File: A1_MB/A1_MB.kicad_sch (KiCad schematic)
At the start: 12 parts, among them J1 Conn_02x04_Counter_Clockwise, J15 Conn_02x04_Odd_Even, J16 USB_A, J2 Screw_Terminal_01x02, U1 Pico

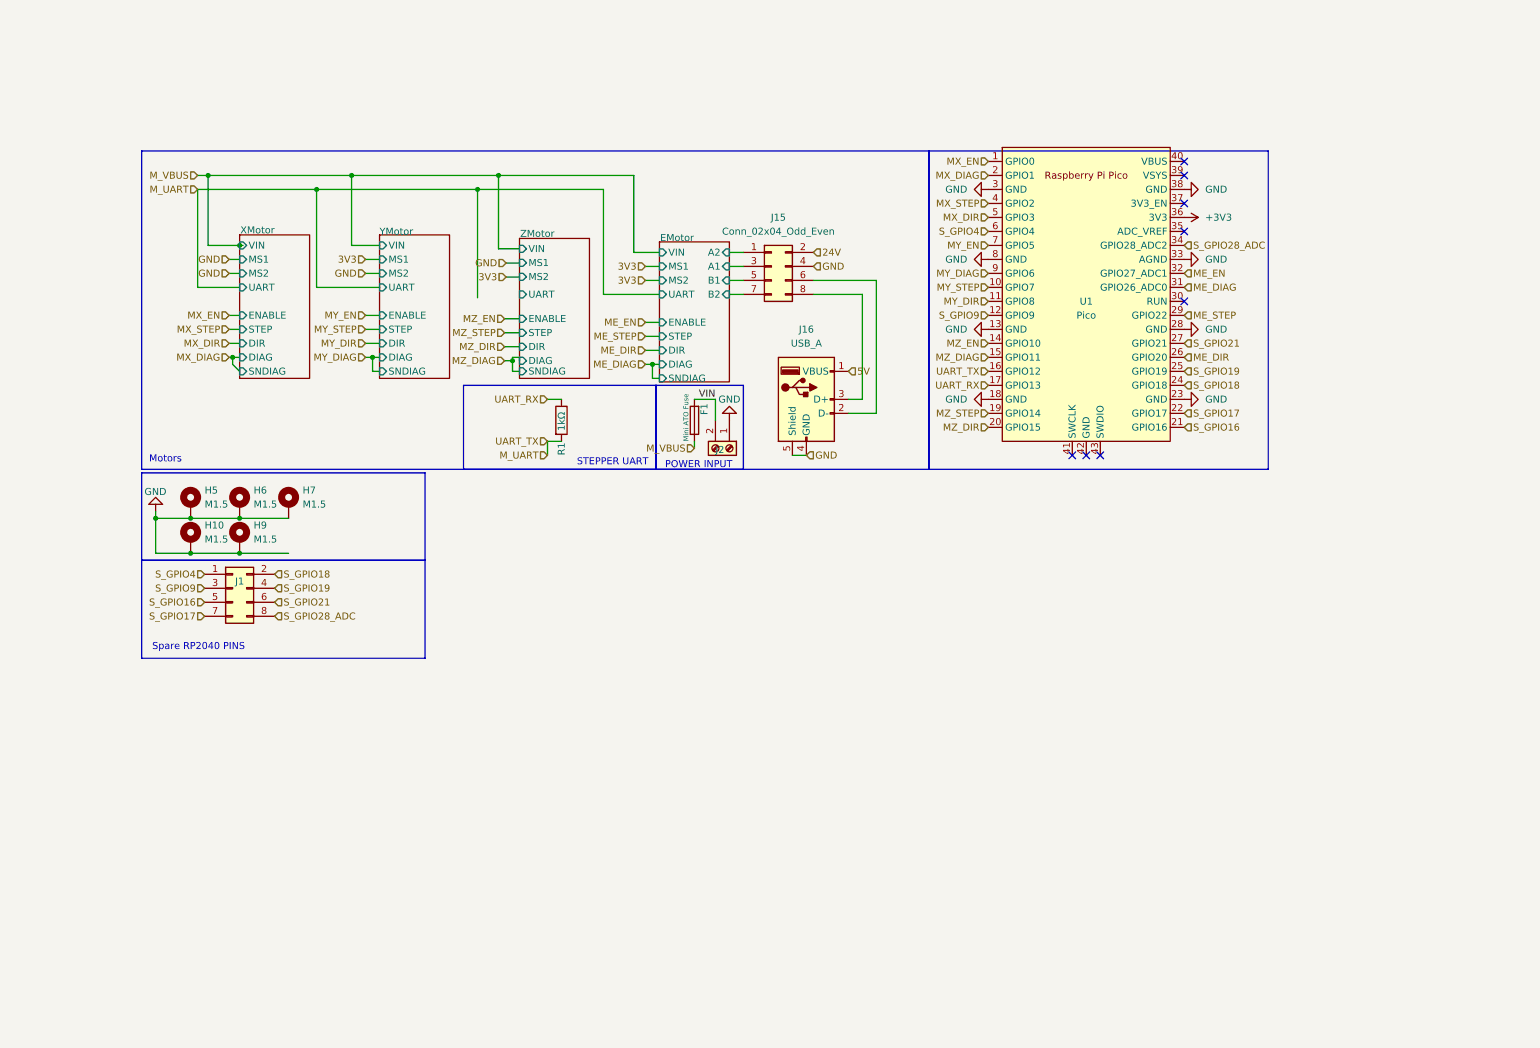
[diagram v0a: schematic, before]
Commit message: e
e
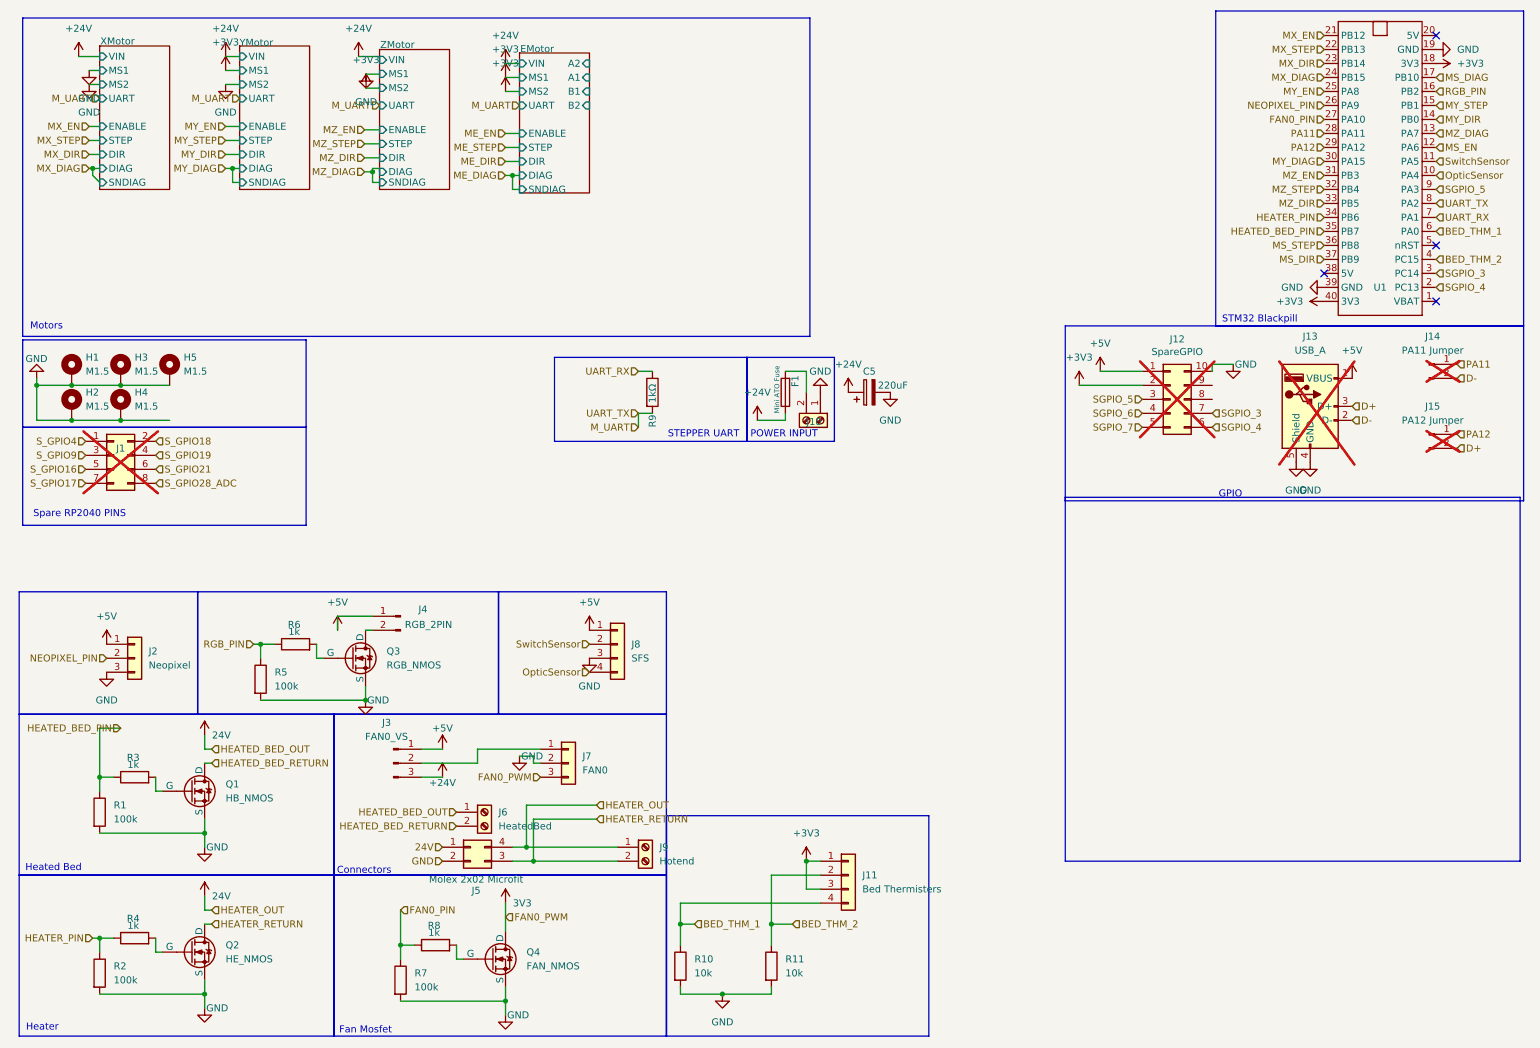
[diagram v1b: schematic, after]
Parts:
- removed J15: Conn_02x04_Odd_Even, symbol Connector_Generic:Conn_02x04_Odd_Even
- removed J16: USB_A, symbol Connector:USB_A
- removed U1: Pico, OpenA1K:Socketed MCU - Pico (No Text), symbol MCU_RaspberryPi_and_Boards:Pico
- added C5: 220uF, Capacitor_THT:CP_Radial_D8.0mm_P3.50mm, symbol Device:C_Polarized
- added J11: Bed Thermisters, Connector_JST:JST_XH_B4B-XH-A_1x04_P2.50mm_Vertical, symbol Connector_Generic:Conn_01x04
- added J12: SpareGPIO, Connector_PinHeader_2.54mm:PinHeader_2x05_P2.54mm_Vertical, symbol Connector_Generic:Conn_02x05_Counter_Clockwise
- added J13: USB_A, Connector_USB:USB3_A_Molex_48393-001, symbol Connector:USB_A
- added J14: PA11 Jumper, Connector_PinHeader_2.54mm:PinHeader_1x02_P2.54mm_Vertical, symbol Connector:Conn_01x02_Pin
- added J15: PA12 Jumper, Connector_PinHeader_2.54mm:PinHeader_1x02_P2.54mm_Vertical, symbol Connector:Conn_01x02_Pin
- added J2: Neopixel, Connector_JST:JST_XH_B3B-XH-AM_1x03_P2.50mm_Vertical, symbol Connector_Generic:Conn_01x03
- added J3: FAN0_VS, Connector_PinHeader_2.54mm:PinHeader_1x03_P2.54mm_Vertical, symbol Connector:Conn_01x03_Pin
- added J4: RGB_2PIN, Connector_JST:JST_XH_B2B-XH-AM_1x02_P2.50mm_Vertical, symbol Connector:Conn_01x02_Pin
- added J5: Molex 2x02 Microfit, Connector_Molex:Molex_Micro-Fit_3.0_43045-0412_2x02_P3.00mm_Vertical, symbol Connector_Generic:Conn_02x02_Counter_Clockwise
- added J6: HeatedBed, OpenA1K:ScrewTerminal 7mm x 7mm, symbol Connector:Screw_Terminal_01x02
- added J7: FAN0, Connector_JST:JST_XH_B3B-XH-AM_1x03_P2.50mm_Vertical, symbol Connector_Generic:Conn_01x03
- added J8: SFS, Connector_JST:JST_XH_B4B-XH-AM_1x04_P2.50mm_Vertical, symbol Connector_Generic:Conn_01x04
- added J9: Hotend, OpenA1K:ScrewTerminal 7mm x 7mm, symbol Connector:Screw_Terminal_01x02
- added Q1: HB_NMOS, OpenA1K:TO254P1054X469X1930-3, symbol Simulation_SPICE:NMOS
- added Q2: HE_NMOS, OpenA1K:TO254P1054X469X1930-3, symbol Simulation_SPICE:NMOS
- added Q3: RGB_NMOS, OpenA1K:TO254P1054X469X1930-3, symbol Simulation_SPICE:NMOS
- added Q4: FAN_NMOS, OpenA1K:TO254P1054X469X1930-3, symbol Simulation_SPICE:NMOS
- added R1, R2, R5, R7: 100k, Resistor_THT:R_Axial_DIN0207_L6.3mm_D2.5mm_P10.16mm_Horizontal, symbol Device:R
- added R10, R11: 10k, Resistor_THT:R_Axial_DIN0207_L6.3mm_D2.5mm_P10.16mm_Horizontal, symbol Device:R
- added R3, R4, R6, R8: 1k, Resistor_THT:R_Axial_DIN0207_L6.3mm_D2.5mm_P10.16mm_Horizontal, symbol Device:R
- added U1: ~, OpenA1K:STM32 Blackpill Socketed, symbol CustomSymbols:STM32F401_Black_Pill
- J1: now not fitted; now left out of the parts list
- renumbered H5 to H1, H10 to H2, H6 to H3, H9 to H4, H7 to H5, J2 to J10, R1 to R9
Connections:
- net +3V3: now also J11.1 (Pin_1), J11.3 (Pin_3), J12.2 (Pin_2), U1.18 (3V3), U1.40 (3V3)
- net 24V: now also J5.1 (Pin_1), J5.4 (Pin_4), J6.1 (Pin_1), J9.1 (Pin_1)
- net 3V3: now also J7.3 (Pin_3), Q4.1 (D)
- net GND: now also C5.2, J12.10 (Pin_10), J13.4 (GND), J13.5 (Shield), J2.3 (Pin_3), J5.2 (Pin_2), J7.2 (Pin_2), J8.3 (Pin_3), Q1.3 (S), Q2.3 (S), Q3.3 (S), Q4.3 (S), R1.2, R10.2, R11.2, R2.2, R5.2, R7.2, U1.19 (GND), U1.39 (GND)
- net MX_DIAG: now also U1.24 (PB15)
- net MX_DIR: now also U1.23 (PB14)
- net MX_EN: now also U1.21 (PB12)
- net MX_STEP: now also U1.22 (PB13)
- net MY_DIAG: now also U1.30 (PA15)
- net MY_DIR: now also U1.14 (PB0)
- net MY_EN: now also U1.25 (PA8)
- net MY_STEP: now also U1.15 (PB1)
- net MZ_DIAG: now also U1.13 (PA7)
- net MZ_DIR: now also U1.33 (PB5)
- net MZ_EN: now also U1.31 (PB3)
- net MZ_STEP: now also U1.32 (PB4)
- net M_UART: now also U1.8 (PA2)
- net UART_RX: now also U1.7 (PA1)
- net M_VBUS renamed +24V
- net +24V: now also C5.1, J3.3 (Pin_3)
- net VIN: no longer names the net of F1.2, J10.2 (Pin_2)
- new net: Q2.2 (G), R4.2
- new net: J3.2 (Pin_2), J7.1 (Pin_1)
- new net: J4.2 (Pin_2), Q3.1 (D)
- new net: Q3.2 (G), R6.2
- new net: Q1.2 (G), R3.2
- new net: Q4.2 (G), R8.2
- new net  HEATED_BED_PIN: R1.1, R3.1
- new net +5V: J12.1 (Pin_1), J13.1 (VBUS), J2.1 (Pin_1), J3.1 (Pin_1), J4.1 (Pin_1), J8.1 (Pin_1)
- new net BED_THM_1: J11.4 (Pin_4), R10.1, U1.6 (PA0)
- new net BED_THM_2: J11.2 (Pin_2), R11.1, U1.4 (PC15)
- new net D+: J13.3 (D+), J15.2 (Pin_2)
- new net D-: J13.2 (D-), J14.2 (Pin_2)
- new net FAN0_PIN: R7.1, R8.1, U1.27 (PA10)
- new net HEATED_BED_PIN: U1.35 (PB7)
- new net HEATED_BED_RETURN: J6.2 (Pin_2), Q1.1 (D)
- new net HEATER_PIN: R2.1, R4.1, U1.34 (PB6)
- new net HEATER_RETURN: J5.3 (Pin_3), J9.2 (Pin_2), Q2.1 (D)
- new net MS_DIAG: U1.17 (PB10)
- new net MS_DIR: U1.37 (PB9)
- new net MS_EN: U1.12 (PA6)
- new net MS_STEP: U1.36 (PB8)
- new net NEOPIXEL_PIN: J2.2 (Pin_2), U1.26 (PA9)
- new net OpticSensor: J8.4 (Pin_4), U1.10 (PA4)
- new net PA11: J14.1 (Pin_1), U1.28 (PA11)
- new net PA12: J15.1 (Pin_1), U1.29 (PA12)
- new net RGB_PIN: R5.1, R6.1, U1.16 (PB2)
- new net SGPIO_3: J12.7 (Pin_7), U1.3 (PC14)
- new net SGPIO_4: J12.6 (Pin_6), U1.2 (PC13)
- new net SGPIO_5: J12.3 (Pin_3), U1.9 (PA3)
- new net SGPIO_6: J12.4 (Pin_4)
- new net SGPIO_7: J12.5 (Pin_5)
- new net SwitchSensor: J8.2 (Pin_2), U1.11 (PA5)
- no-connect marks 8 -> 4
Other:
- note added: "Connectors"
- note added: "Fan Mosfet"
- note added: "GPIO"
- note added: "Heated Bed"
- note added: "Heater"
- note added: "STM32 Blackpill"
- moved on the sheet: F1, H1, H2, H3, H4, H5, J10, R9
